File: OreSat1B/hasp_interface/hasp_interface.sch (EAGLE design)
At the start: 79 parts, among them J1 SAMTEC-MMS-104-02-X-SHJ, J2 ORESAT-DEBUG-CONNECTOR-ALL, Q1 MMBT2907SMD, U1 TCAN330, U10 TPS63070, U2 LM60440ARPKR, U7 STM32F091C, X1 16MHZ-2.5x2mm

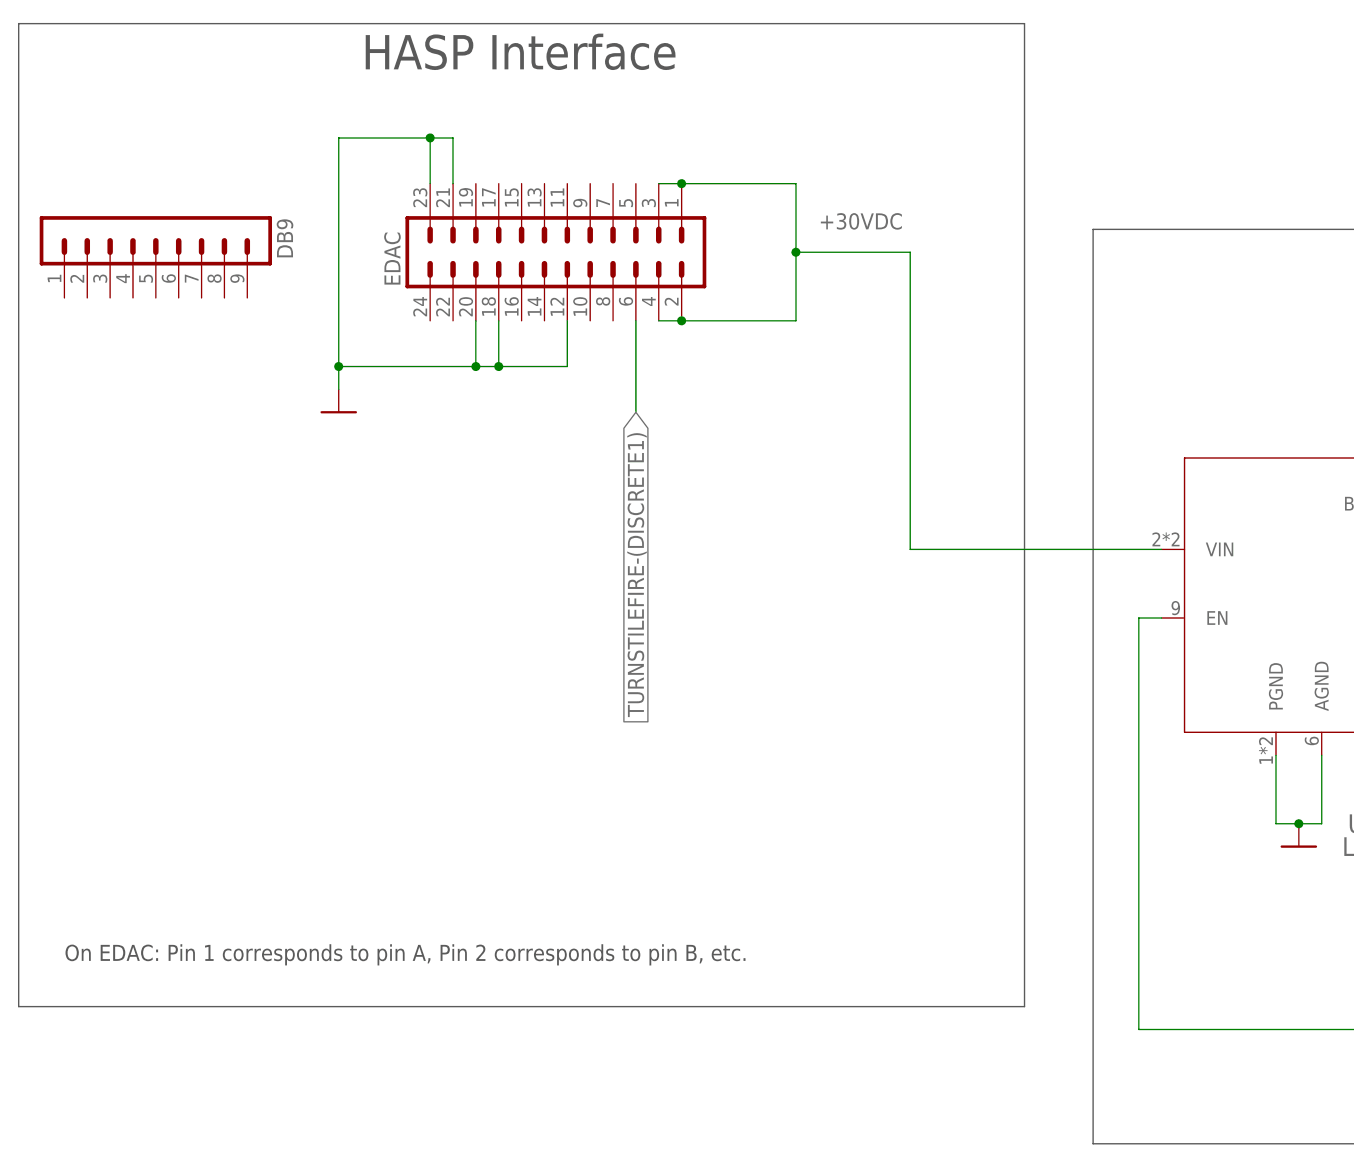
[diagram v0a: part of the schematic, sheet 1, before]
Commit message: Wire cleanup
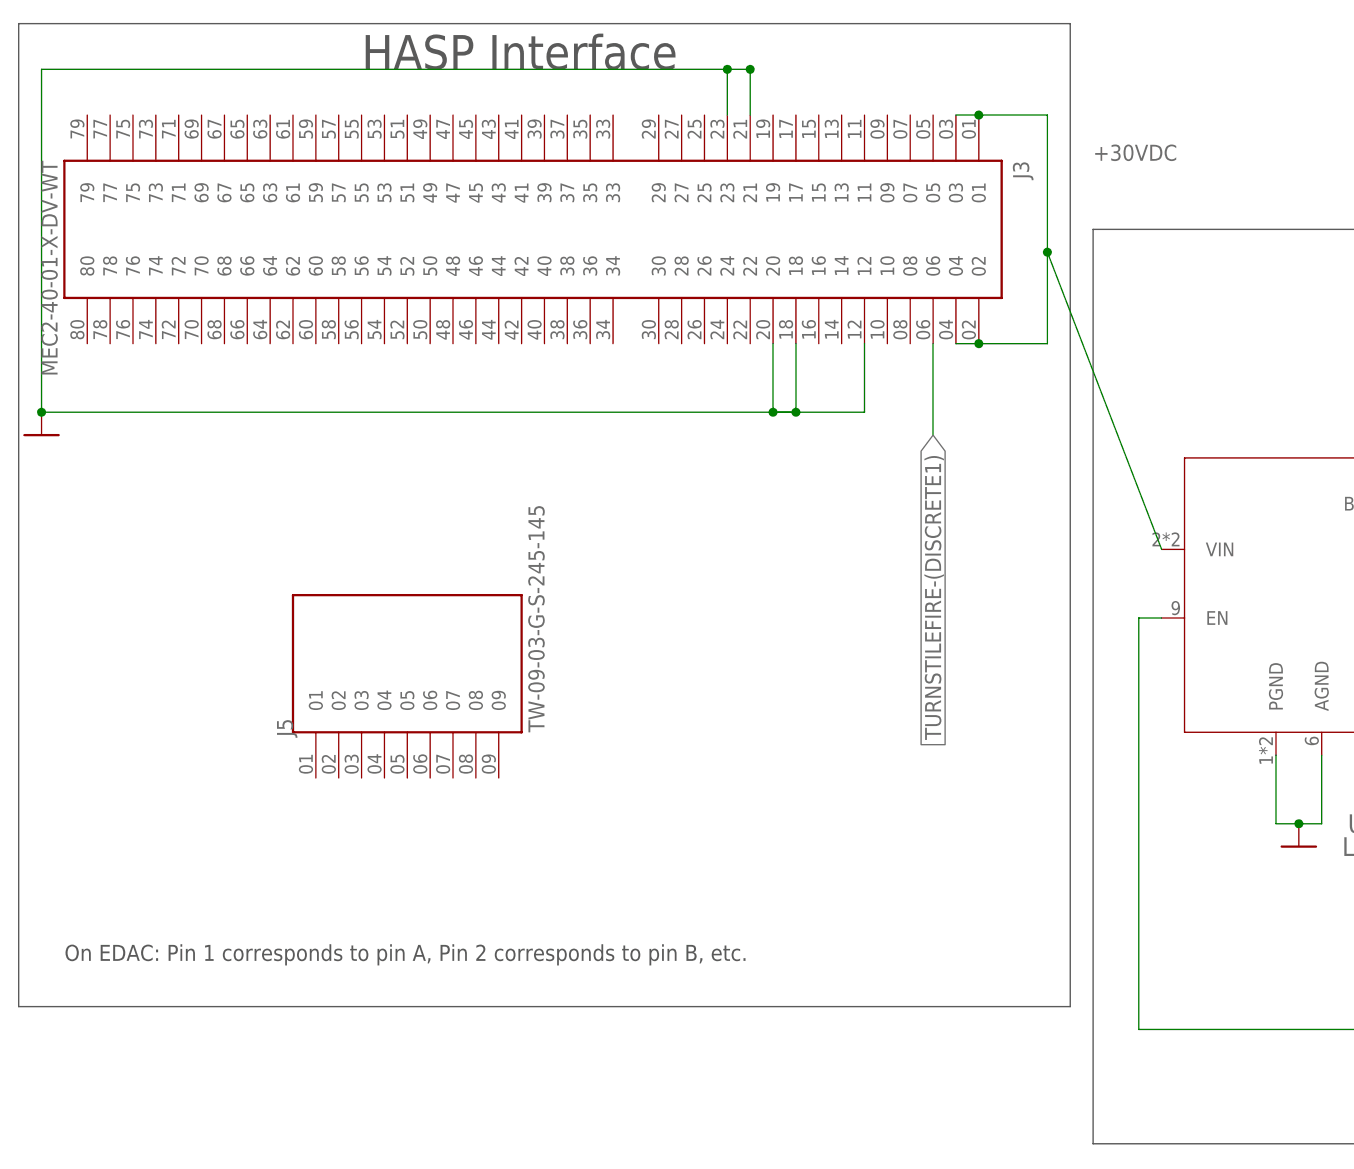
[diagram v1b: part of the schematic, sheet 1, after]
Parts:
- removed DB9: (no value), con-lstb:MA09-1
- removed EDAC: (no value), con-lstb:MA12-2
- added J3: MEC2-40-01-X-DV-WT, MEC2-40-01-X-DV-WT:MEC2-40-01-X-DV-WT
- added J5: TW-09-03-G-S-245-145, TW-09-03-G-S-245-145:TW-09-03-G-S-245-145
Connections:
- net +30VDC: now also J3.01, J3.02, J3.03, J3.04; no longer EDAC.1, EDAC.2, EDAC.3, EDAC.4
- net GND: now also J3.12, J3.18, J3.20, J3.21, J3.23; no longer EDAC.12, EDAC.18, EDAC.20, EDAC.21, EDAC.23
- net TURNSTILEFIRE-(DISCRETE1): now also J3.06; no longer EDAC.6
